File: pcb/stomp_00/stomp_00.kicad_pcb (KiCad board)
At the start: 2 copper layers, 54 x 106 mm, 49 parts, among them J1 9V_Power_Input, J10 AudioJack3, J11 AudioJack3, J2 Conn_01x09, J3 GuitarInput1, J4 Headphones, J5 GuitarOutput1, J6 Conn_01x09, J7 Conn_02x04_Counter_Clockwise, SW1 SW_DIP_x04, SW2 Footswitch, U1 AP7313-18SAG, U14 6N138, U2 TL072, U4 XL1509-5.0, U7 Teensy4.1, U9 SGTL5000XNAA3

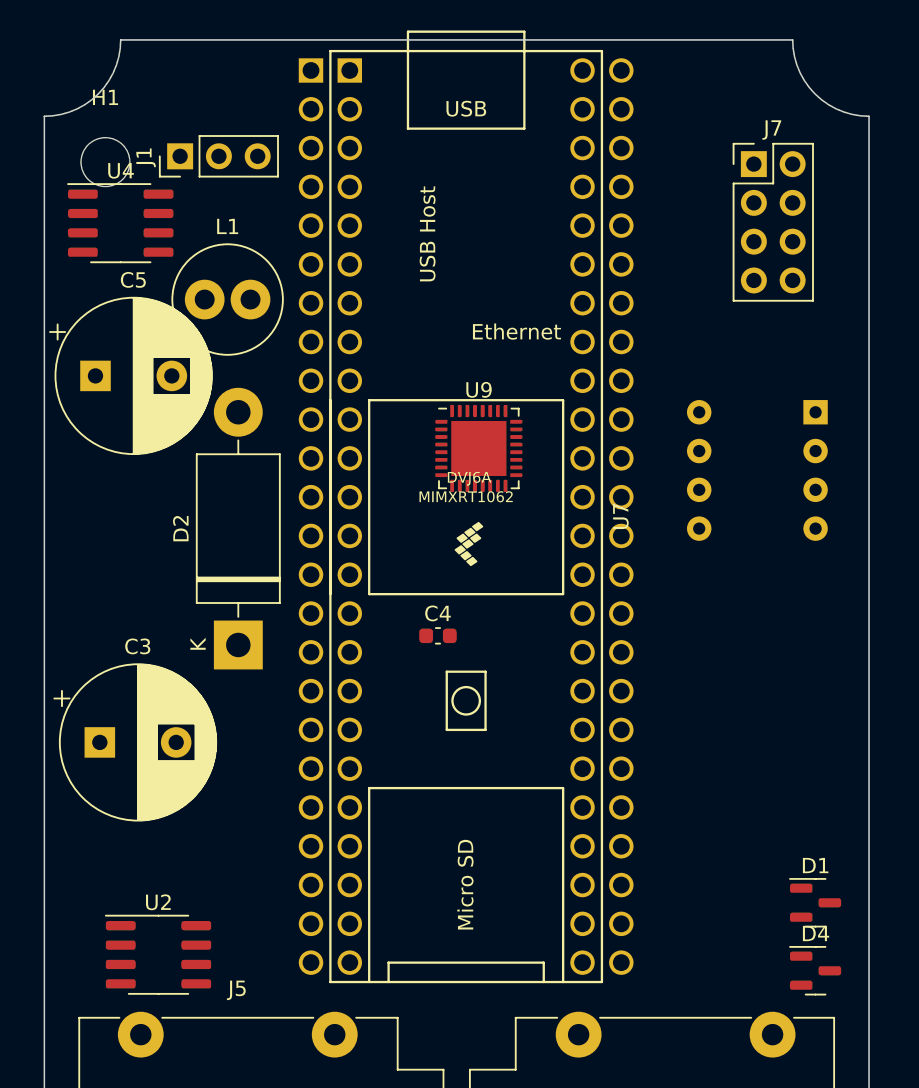
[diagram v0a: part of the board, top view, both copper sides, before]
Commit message: 9v power stuff
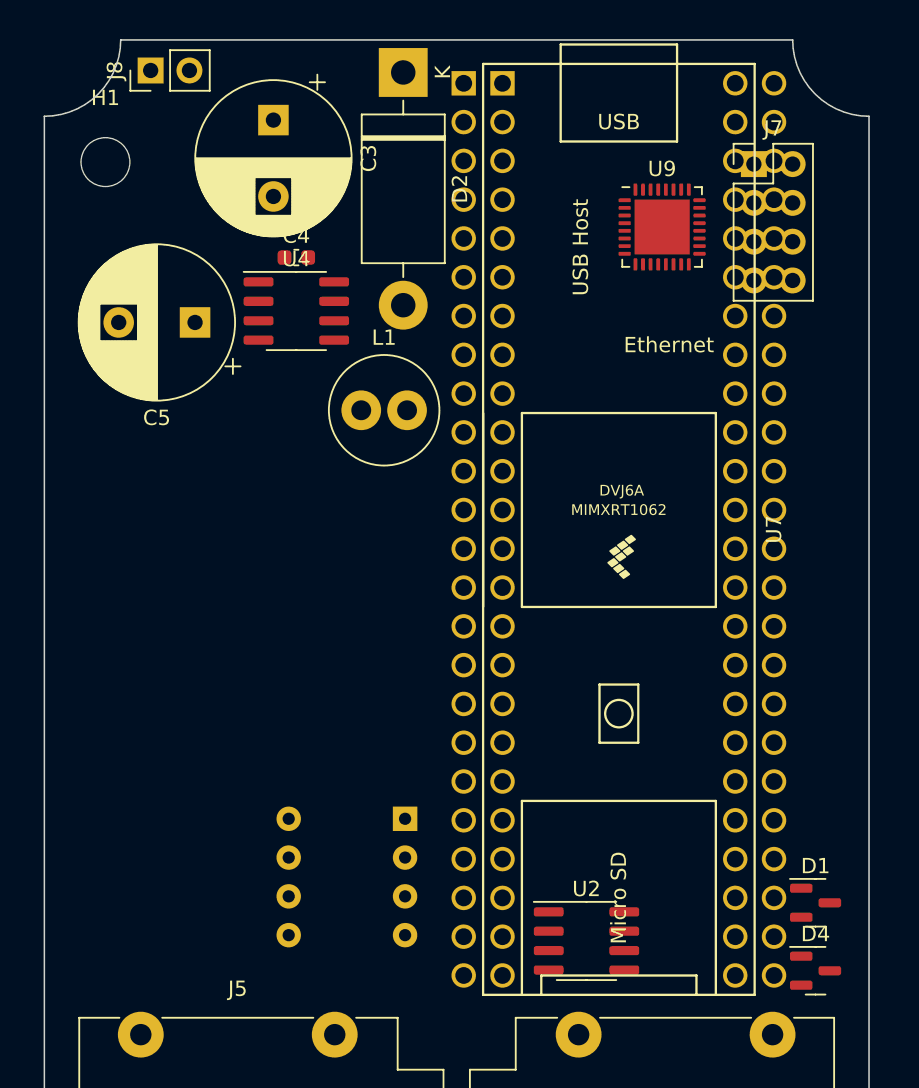
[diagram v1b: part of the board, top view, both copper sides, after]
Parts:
- removed J1: 9V_Power_Input, Connector_PinHeader_2.54mm:PinHeader_1x03_P2.54mm_Vertical
- added J8: Barrel_Jack, Connector_PinHeader_2.54mm:PinHeader_1x02_P2.54mm_Vertical, F.Cu at (6.96, 2.00)
- moved C3 42.3 mm to (15.0, 5.25), turned to -90 degrees
- moved D2 39.0 mm to (23.5, 2.13), turned to -90 degrees
- moved SW1 37.8 mm to (23.6, 51.0)
- moved U2 28.0 mm to (35.5, 59.0)
- moved C4 26.4 mm to (16.5, 14.2)
- moved U9 18.8 mm to (40.5, 12.2)
- moved U4 12.9 mm to (16.5, 17.8)
- moved L1 12.6 mm to (20.8, 24.2)
- moved U7 10.0 mm to (37.6, 32.0)
- moved C5 7.40 mm to (9.87, 18.5), turned to 180 degrees
